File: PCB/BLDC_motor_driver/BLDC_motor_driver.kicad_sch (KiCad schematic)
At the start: 14 parts, among them U10 AS5048A, U5 SN65HVD230, U6 STM32F405RGTx, Y1 8MHz

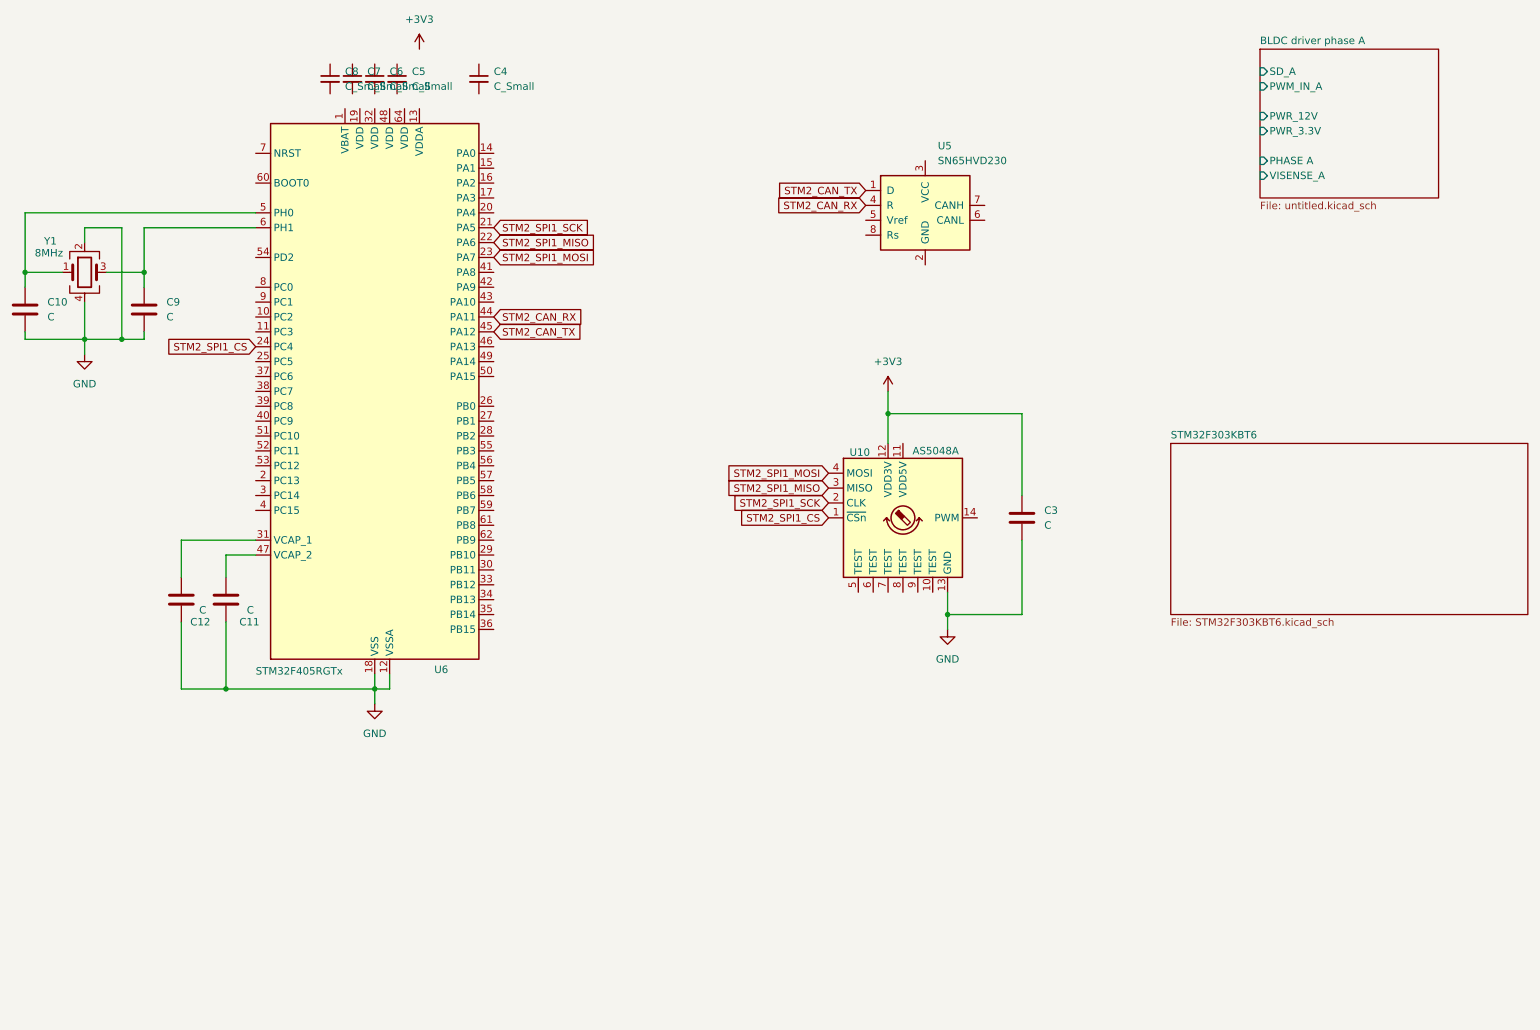
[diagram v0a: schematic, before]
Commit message: updated schematic
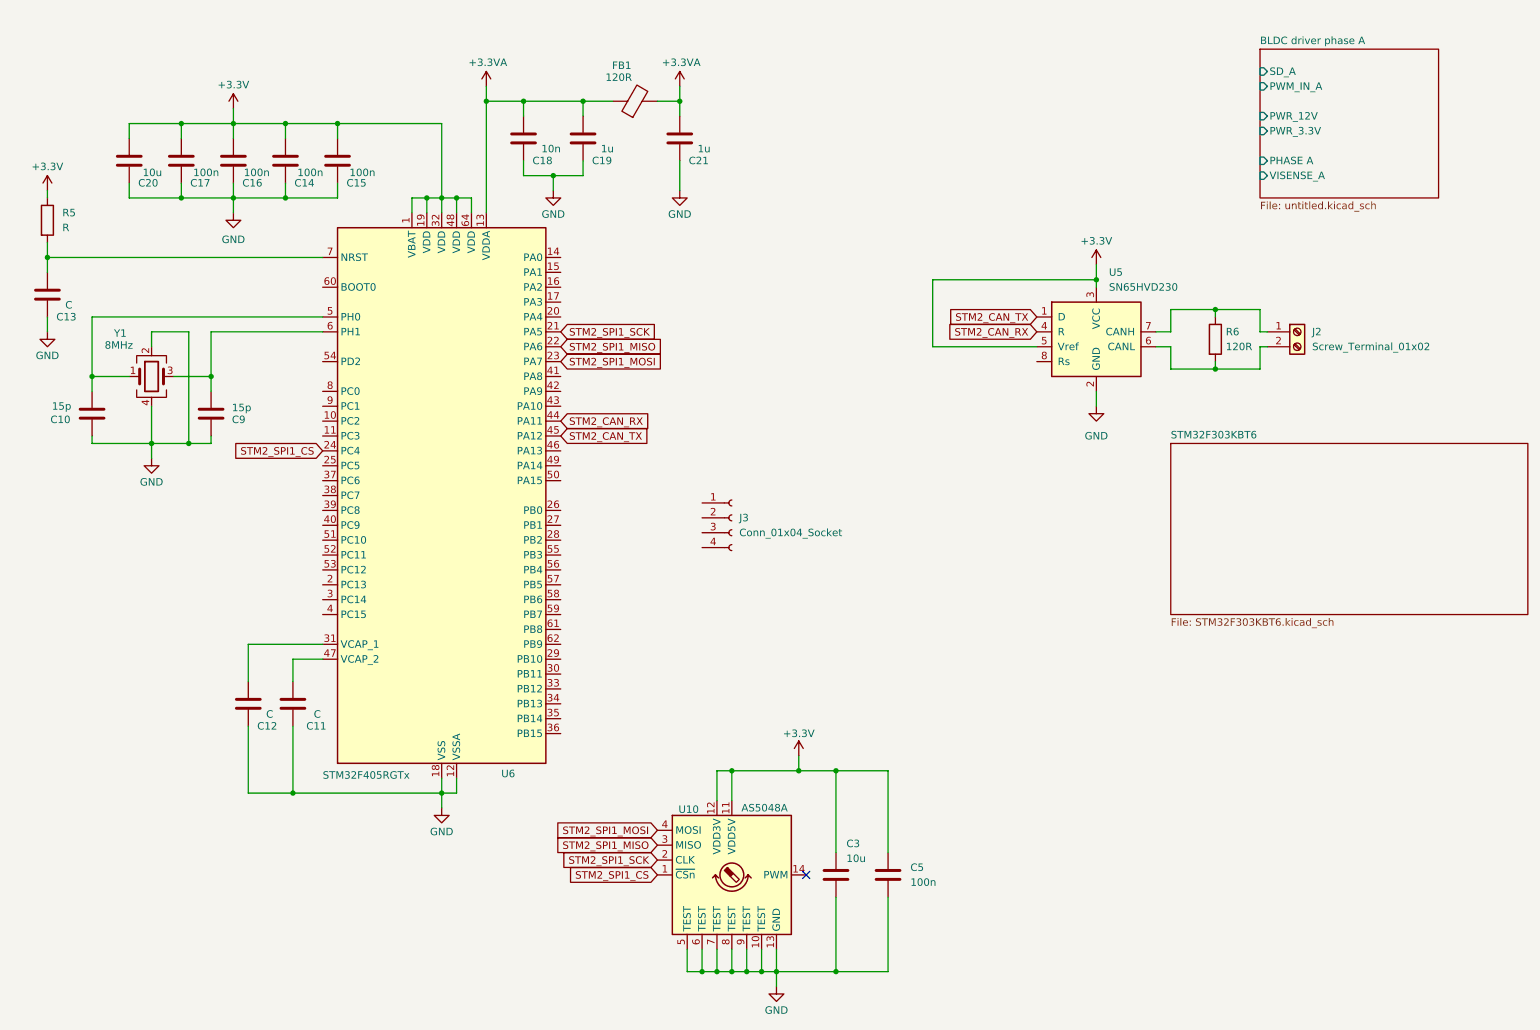
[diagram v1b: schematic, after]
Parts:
- removed C4, C5, C6, C7, C8: C_Small, symbol Device:C_Small
- added C13: C, symbol Device:C
- added C14, C15, C16, C17: 100n, symbol Device:C
- added C18: 10n, symbol Device:C
- added C19, C21: 1u, symbol Device:C
- added C20: 10u, symbol Device:C
- added C5: 100n, Capacitor_SMD:C_0504_1310Metric, symbol Device:C
- added FB1: 120R, symbol Device:FerriteBead
- added J2: Screw_Terminal_01x02, TerminalBlock:TerminalBlock_Xinya_XY308-2.54-2P_1x02_P2.54mm_Horizontal, symbol Connector:Screw_Terminal_01x02
- added J3: Conn_01x04_Socket, Connector_PinHeader_2.54mm:PinHeader_1x04_P2.54mm_Vertical, symbol Connector:Conn_01x04_Socket
- added R5: R, symbol Device:R
- added R6: 120R, Resistor_SMD:R_0402_1005Metric, symbol Device:R
- C10, C9: value C -> 15p; footprint (none) -> Capacitor_SMD:C_0603_1608Metric
- C3: value C -> 10u; footprint (none) -> Capacitor_SMD:C_0504_1310Metric
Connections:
- net +3V3 is gone; now on net +3.3V: C3.1, U10.12 (VDD3V)
- net GND: now also C10.1, U10.10 (TEST), U10.5 (TEST), U10.6 (TEST), U10.7 (TEST), U10.8 (TEST), U10.9 (TEST), U5.2 (GND), C13.2, C14.2, C15.2, C16.2, C17.2, C18.2, C19.2, C20.2, C21.2, C5.2; no longer C10.2
- net at U6.5 (PH0), Y1.1: now also C10.2; no longer C10.1
- net +3.3V: now reaches U5.3 (VCC)
- net +3.3V: now also U10.11 (VDD5V), U5.5 (Vref), U6.1 (VBAT), U6.19 (VDD), U6.32 (VDD), U6.48 (VDD), U6.64 (VDD), C14.1, C15.1, C16.1, C17.1, C20.1, C5.1, R5.1
- net at U5.6 (CANL): now also J2.2 (Pin_2), R6.2
- net at U5.7 (CANH): now also J2.1 (Pin_1), R6.1
- net +3.3VA: now reaches U6.13 (VDDA)
- net +3.3VA: now also C18.1, C19.1, C21.1, FB1.1, FB1.2
- net at U6.7 (NRST): now also C13.1, R5.2
- no-connect marks 0 -> 1
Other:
- moved on the sheet: C10, C11, C12, C3, C9, U10, U5, U6, Y1
